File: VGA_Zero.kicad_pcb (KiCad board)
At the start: 2 copper layers, 65 x 30 mm, 33 parts, among them J1 VGA, J2 CONN_02X20, J3 AUDIO, J4 SPI, J5 BARREL_JACK

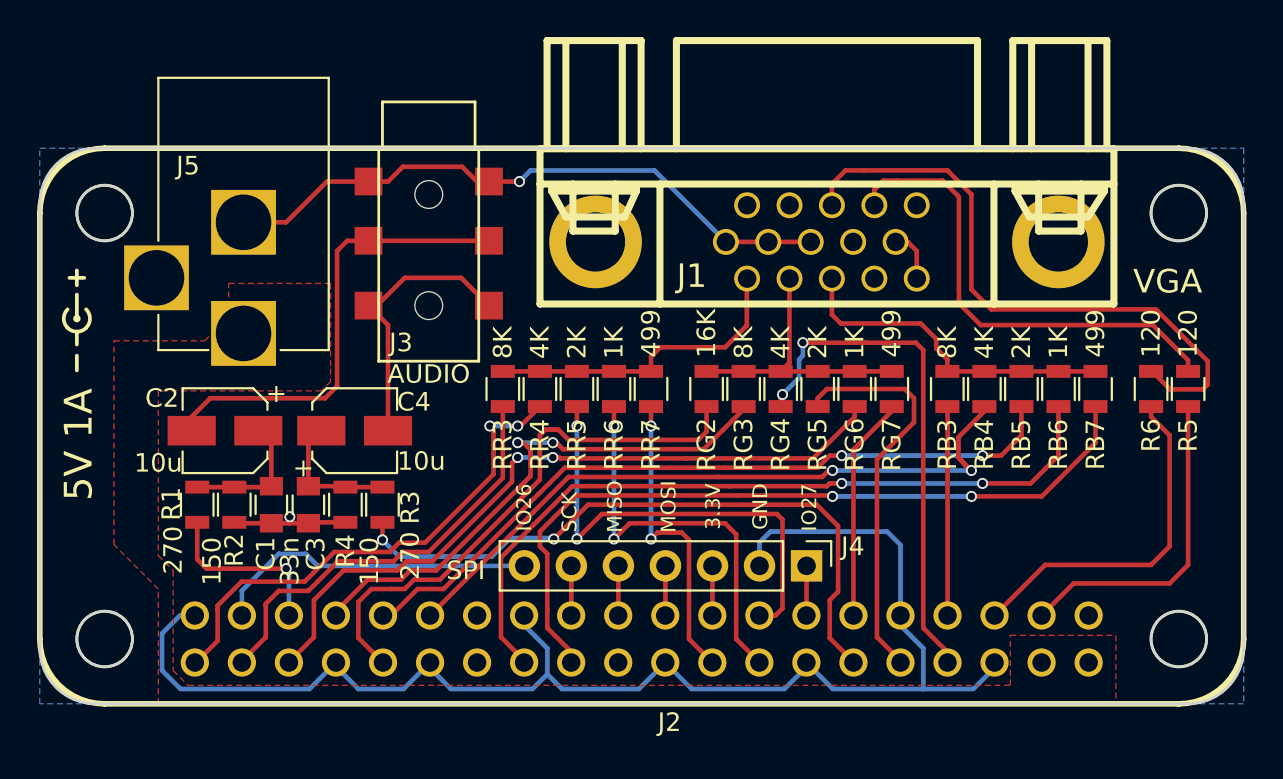
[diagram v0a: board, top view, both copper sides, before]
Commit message: rev3
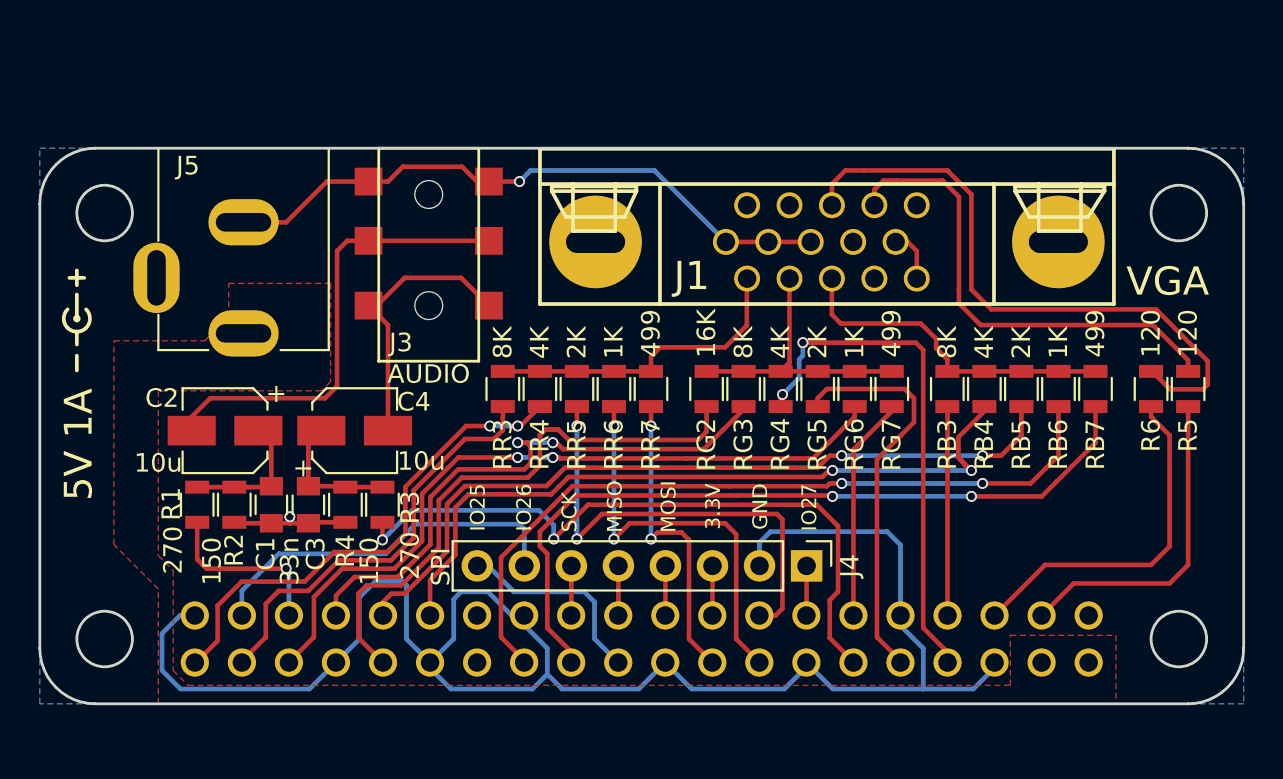
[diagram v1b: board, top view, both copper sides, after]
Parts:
- J4: footprint Pin_Headers:Pin_Header_Straight_1x07_Pitch2.54mm -> Pin_Headers:Pin_Header_Straight_1x08_Pitch2.54mm
- J5: footprint Connectors:BARREL_JACK -> _LaurentPerso:BARREL_JACK
- moved REF*** 0.81 mm to (40.4, 35.0)
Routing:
- net GND: track 121.2 -> 135.0 mm
- net /IO25: track 0.00 -> 10.9 mm
- net /B4: track 37.8 -> 40.4 mm
- net /IO26: track 17.7 -> 20.2 mm
- net /B5: track 40.2 -> 42.1 mm
- net /G2: track 30.1 -> 31.5 mm
- net /G6: track 38.6 -> 39.6 mm
- net /RPWM: track 35.8 -> 36.8 mm
- net /G3: track 30.9 -> 31.7 mm
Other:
- board text added: "Desingned by Laurent Le Goff (2017) http://github.com/llegoff/VGA_Zero Use dtoverlay vga565 with parameter dpi_output_format=0x13 For Audio dtoverlay=pwm-2chan,pin=18,func=2,pin2=19,func2=2"
- board text added: "IO25"
- board text removed: "Desingned by Laurent Le Goff (2017) http://github.com/llegoff/VGA_Zero Use dtoverlay dpi24 with parameter dpi_output_format=0x13 For Audio & SPI, remake dpi24.dtbo without pin GPIO 9 10 11 18 19 25 26 27 dtoverlay=pwm-2chan,pin=18,func=2,pin2=19,func2=2"
